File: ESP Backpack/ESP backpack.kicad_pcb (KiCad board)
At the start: 2 copper layers, 100 x 100 mm, 33 parts, among them J1 HLE-120-02-F-DV-BE-K, J2 HLE-120-02-F-DV-BE-K, U1 ESP32-DEVKITC-32D, U2 VCNL4010-GS08

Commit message: edit weird fill issue
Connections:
- J1 pad 30: Net-(J1-Pad30) -> GND
- J1 pad 34: Net-(J1-Pad34) -> GND
- J1 pad 38: Net-(J1-Pad38) -> GND
- J2 pad 29: Net-(J2-Pad29) -> +5V
- J2 pad 30: Net-(J2-Pad30) -> GND
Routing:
- net Net-(J1-Pad34): track 1.41 -> 0.00 mm
- net GND: track 28.5 -> 29.9 mm

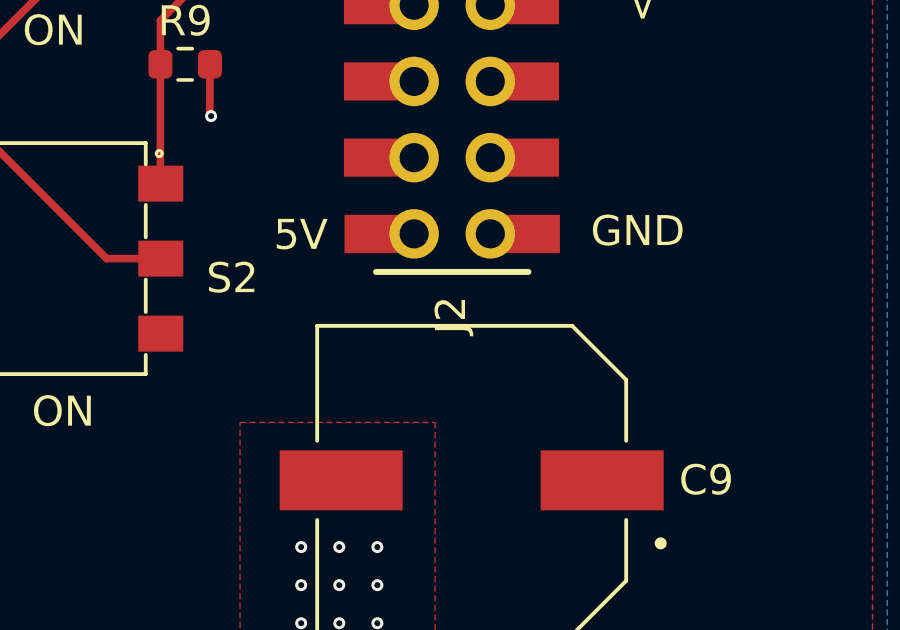
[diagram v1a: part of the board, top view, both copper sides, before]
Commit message: reorg to more standard file tree
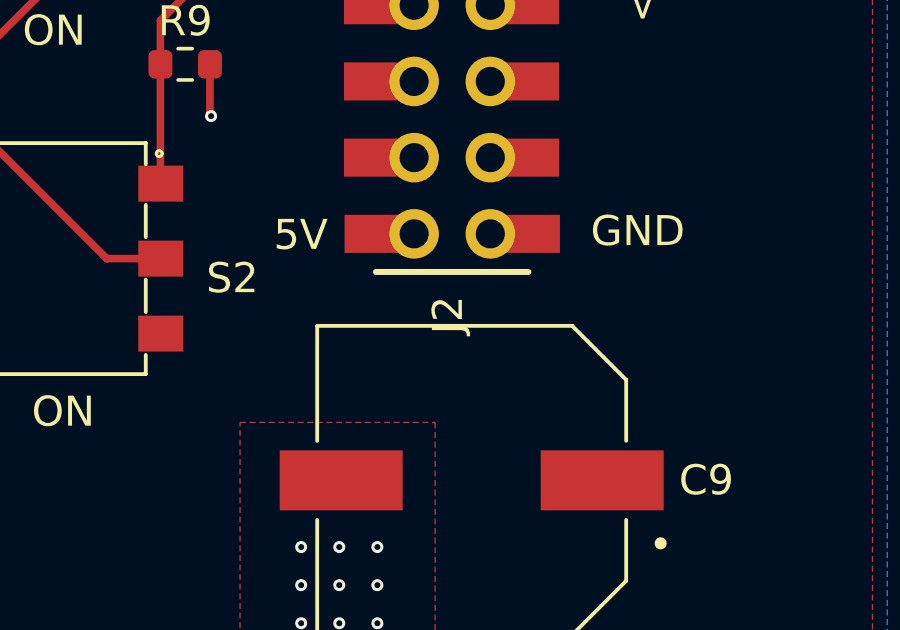
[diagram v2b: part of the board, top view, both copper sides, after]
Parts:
- D1: footprint LED_SK6812 -> _ESP-Backpack-Custom-Libraries:LED_SK6812
- J1, J2: footprint Custom Libraries:SAMTEC_HLE-120-02-F-DV-BE-K -> _ESP-Backpack-Custom-Libraries:SAMTEC_HLE-120-02-F-DV-BE-K
- S1, S2: footprint 452403012014 -> _ESP-Backpack-Custom-Libraries:452403012014
- U1: footprint Custom Libraries:MODULE_ESP32-DEVKITC-32D -> _ESP-Backpack-Custom-Libraries:MODULE_ESP32-DEVKITC-32D
- U2: footprint Custom Libraries:XDCR_VCNL4010-GS08 -> _ESP-Backpack-Custom-Libraries:XDCR_VCNL4010-GS08
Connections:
- J1 pad 30: GND -> Net-(J1-Pad30)
- J1 pad 34: GND -> Net-(J1-Pad34)
- J1 pad 38: GND -> Net-(J1-Pad38)
- J2 pad 29: +5V -> Net-(J2-Pad29)
- J2 pad 30: GND -> Net-(J2-Pad30)
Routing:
- net Net-(J1-Pad34): track 0.00 -> 1.41 mm
- net GND: track 29.9 -> 28.5 mm
